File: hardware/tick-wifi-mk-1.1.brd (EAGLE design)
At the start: 100 x 64 mm, 33 parts, among them IC1 MAX7219, IC2 MAX7219, IC3 74HC125, IC4 LD1117 5V, U1 Adafruit Feather HUZZAH ESP82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

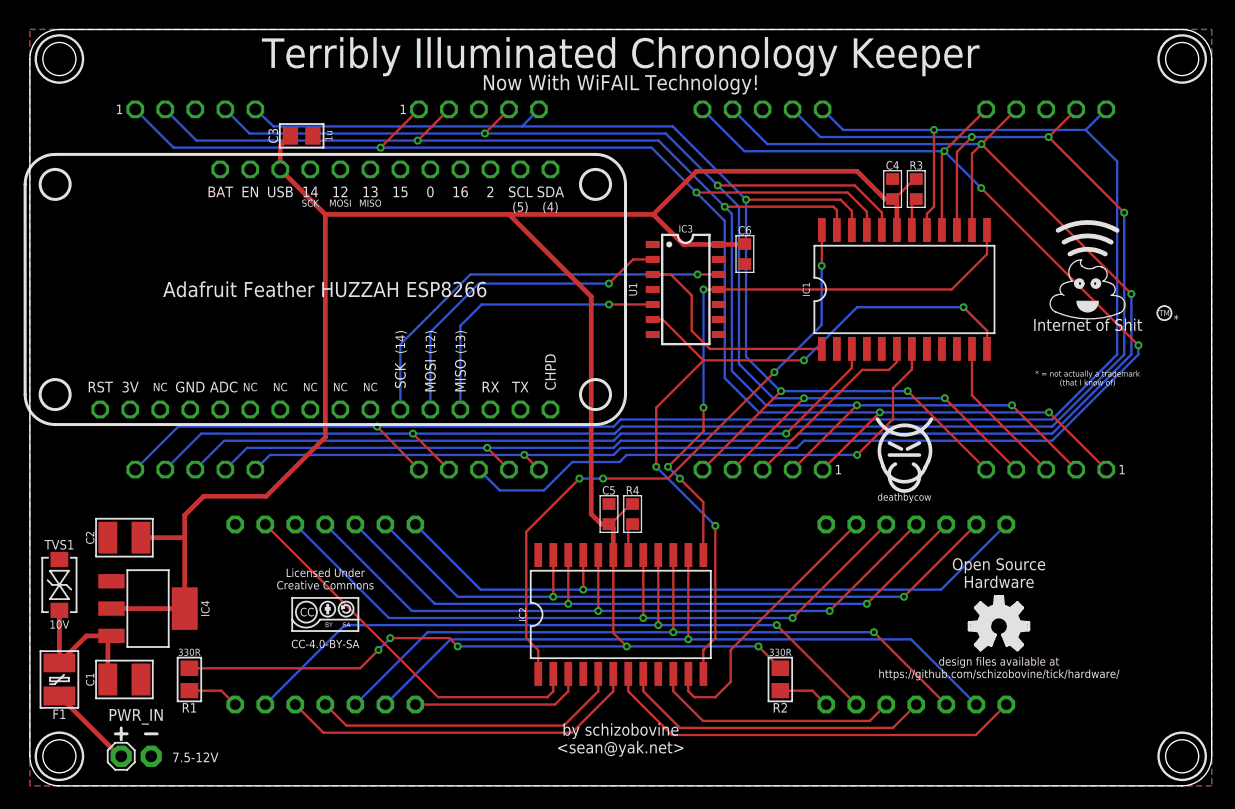
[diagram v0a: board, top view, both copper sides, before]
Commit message: more wip
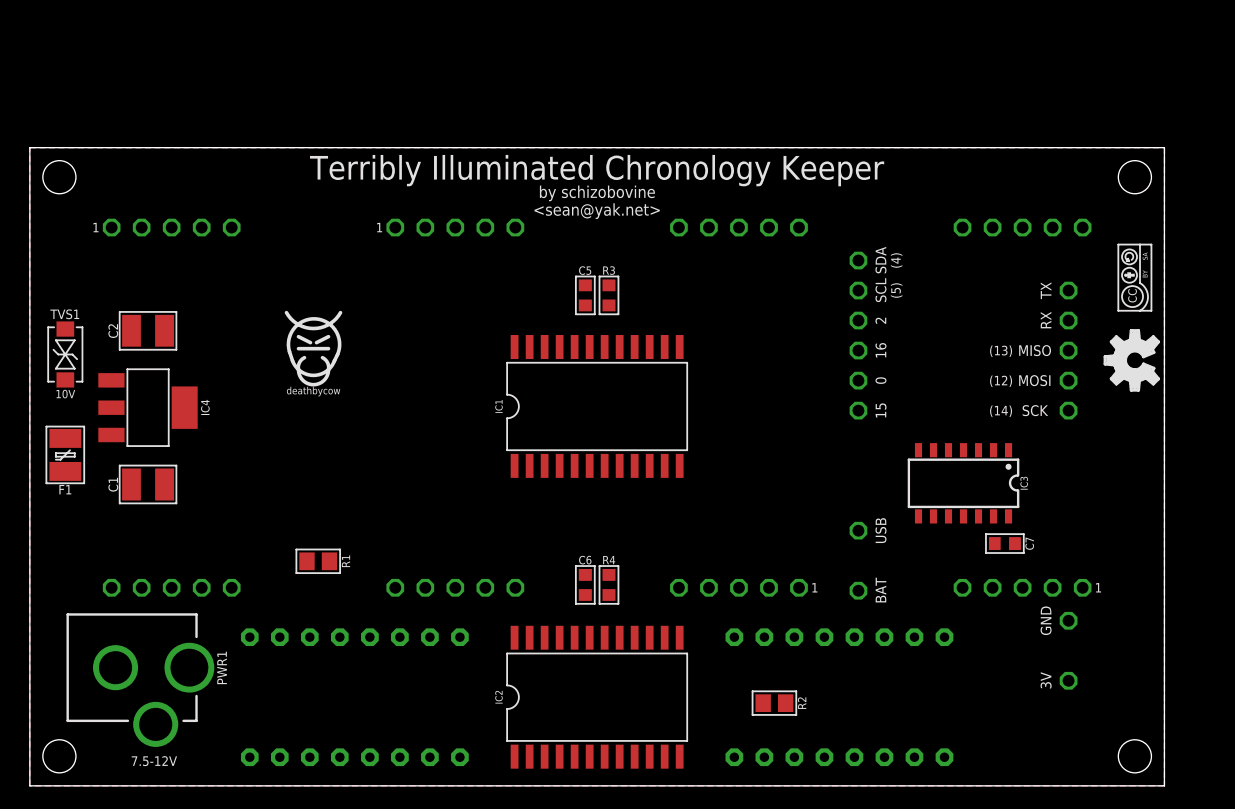
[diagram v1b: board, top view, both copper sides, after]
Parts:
- removed C3: 1u, a_parts:C0805
- removed C4: 100n, a_parts:C0603
- removed PWR_IN: M02PTH-CENTERED-R+, A_butts:1X02-CENTER-R+
- removed U$5: (no value), a_parts:OSHWLOGO_TINY_SILKONLY
- removed U$6: (no value), A_butts:CC-BY-SA-4.0-NO-URL
- removed U$7, U$8: (no value), a_parts:INTERNET_OF_SHIT
- added C7: 100n, a_parts:C0603
- added PWR1: DCBARRELPTH, a_parts:DCJACK_2MM_PTH
- DIGIT1, DIGIT2, DIGIT3, DIGIT4: device A_butts:7SEG_1DIG_25.4MM_NOSILK -> a_parts:7SEG_1DIG_25.4MM_NOSILK
- DISPLAY1, DISPLAY2: value 7SEG_4DIGIT_COLON14.2MM-CC -> 7SEG_4DIGIT_COLON_APOS; device a_parts:7SEG_4DIG_0.56IN_14MM_ADAFRUIT -> a_parts:7SEG_4DIG_10MM
- F1: device A_butts:PTC-1210 -> a_parts:PTC-1210
- FRAME1: device A_butts:DUMMY -> a_parts:DUMMY
- TVS1: device A_butts:SMA-DIODE-TVS-BIDIR -> a_parts:SMA-DIODE-TVS-BIDIR
- U$1: device A_butts:TICK_SYMBOL -> a_parts:TICK_SYMBOL
- U$2: device A_butts:COW_SMALL -> a_parts:COW_SMALL
- U$4: device A_butts:CC-BY-SA-4.0-NO-URL -> a_parts:CC-BY-SA-4.0-NO-URL
- U1: value Adafruit Feather HUZZAH ESP8266 -> ADAFRUIT_FEATHER_HUZZAH_ESP8266_TICK; device a_parts:ADAFRUIT_FEATHER_HUZZAH -> a_parts:ADAFRUIT_FEATHER_HUZZAH_TICK
- moved U$4 74.2 mm to (93.5, 43.0), turned to 90 degrees
- moved U1 56.5 mm to (79.0, 25.4), turned to 90 degrees
- moved U$2 50.8 mm to (24.0, 37.5)
- moved C6 31.1 mm to (47.0, 17.0)
- moved IC3 28.7 mm to (79.0, 25.6), turned to 180 degrees
- moved IC1 27.8 mm to (48.0, 32.1)
- moved R3 27.5 mm to (49.0, 41.5)
- moved U$3 25.3 mm to (93.5, 36.0), turned to 90 degrees
- moved TVS1 19.5 mm to (3.00, 36.5)
- moved F1 19.0 mm to (3.00, 28.0)
- moved C5 18.6 mm to (47.0, 41.5)
- moved C2 17.6 mm to (10.0, 38.5)
- moved IC4 17.0 mm to (10.0, 32.0)
- moved C1 16.6 mm to (10.0, 25.5)
- moved R1 14.8 mm to (24.4, 19.0), turned to 180 degrees
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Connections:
- net 5V: now also C6.2, C7.1; no longer C3.1, C4.2, C6.1
- net DIG_10: now also DISPLAY2.2, IC2.10; no longer DISPLAY2.P$11, IC2.8
- net DIG_11: now also DISPLAY2.6, IC2.5; no longer DISPLAY2.P$10, IC2.10
- net DIG_12: now also DISPLAY2.8, IC2.8; no longer DISPLAY2.P$6, IC2.11
- net DIG_5: now also DISPLAY1.1, IC2.2; no longer DISPLAY1.P$14, IC2.3
- net DIG_6: now also DISPLAY1.2, IC2.11; no longer DISPLAY1.P$11, IC2.5
- net DIG_7: now also DISPLAY1.6; no longer DISPLAY1.P$10
- net DIG_8: now also DISPLAY1.8, IC2.7; no longer DISPLAY1.P$6, IC2.2
- net DIG_9: now also DISPLAY2.1, IC2.3; no longer DISPLAY2.P$14, IC2.7
- net GND: now also C6.1, C7.2, DISPLAY1.12, DISPLAY2.12, PWR1.BRK; no longer C3.2, C4.1, C6.2, DISPLAY1.P$7, DISPLAY2.P$7, PWR_IN.1
- net N$1: now also PWR1.PWR; no longer PWR_IN.2
- net N$3: now also DISPLAY1.4; no longer DISPLAY1.P$8
- net N$5: now also DISPLAY2.4; no longer DISPLAY2.P$8
- net SEG_2A: now also DISPLAY1.14, DISPLAY2.14; no longer DISPLAY1.P$13, DISPLAY2.P$13
- net SEG_2B: now also DISPLAY1.16, DISPLAY2.16; no longer DISPLAY1.P$9, DISPLAY2.P$9
- net SEG_2C: now also DISPLAY1.13, DISPLAY2.13; no longer DISPLAY1.P$4, DISPLAY2.P$4
- net SEG_2D: now also DISPLAY1.3, DISPLAY2.3; no longer DISPLAY1.P$2, DISPLAY2.P$2
- net SEG_2E: now also DISPLAY1.5, DISPLAY2.5; no longer DISPLAY1.P$1, DISPLAY2.P$1
- net SEG_2F: now also DISPLAY1.11, DISPLAY2.11; no longer DISPLAY1.P$12, DISPLAY2.P$12
- net SEG_2G: now also DISPLAY1.15, DISPLAY2.15; no longer DISPLAY1.P$5, DISPLAY2.P$5
- net SEG_2P: now also DISPLAY1.7, DISPLAY2.7; no longer DISPLAY1.P$3, DISPLAY2.P$3
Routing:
- net 5V: track 220.5 -> 0.00 mm, vias 5 -> 0
- net SEG_1G: track 146.5 -> 0.00 mm, vias 2 -> 0
- net SEG_1F: track 144.9 -> 0.00 mm, vias 4 -> 0
- net SEG_1A: track 140.4 -> 0.00 mm, vias 3 -> 0
- net SEG_1B: track 138.2 -> 0.00 mm, vias 4 -> 0
- net SEG_1E: track 130.6 -> 0.00 mm, vias 4 -> 0
- net SEG_1D: track 120.2 -> 0.00 mm, vias 4 -> 0
- net SEG_1C: track 115.1 -> 0.00 mm, vias 4 -> 0
- net SEG_1P: track 104.6 -> 0.00 mm, vias 3 -> 0
- net DISP_LOAD: track 64.6 -> 0.00 mm, vias 4 -> 0
- net SEG_2G: track 61.9 -> 0.00 mm, vias 2 -> 0
- net SEG_2A: track 61.7 -> 0.00 mm, vias 1 -> 0
- net SEG_2F: track 61.6 -> 0.00 mm, vias 2 -> 0
- net SEG_2B: track 61.5 -> 0.00 mm, vias 2 -> 0
- net SEG_2C: track 60.8 -> 0.00 mm, vias 2 -> 0
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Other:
- board size 100 x 64 mm -> 96 x 54 mm
- board text removed: "*"
- board text removed: "* = not actually a trademark (that I know of)"
- board text removed: "CC-4.0-BY-SA"
- board text removed: "Internet of Shit"
- board text removed: "Licensed Under Creative Commons"
- board text removed: "Open Source Hardware"
- board text removed: "TM"
- board text removed: "design files available at https://github.com/schizobovine/tick/hardware/"
